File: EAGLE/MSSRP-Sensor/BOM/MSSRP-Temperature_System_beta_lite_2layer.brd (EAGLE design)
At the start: 50 x 75 mm, 54 parts, among them J1 POWER_JACKPTH, J4 TE-2-TERMBLOCK, J5 TE-2-TERMBLOCK, U1 MBED, U12 LP2989AIM, U2 BLUETOOTH-RN41", U5 SI7020-A10, U7 MAX6675, U8 MAX6675

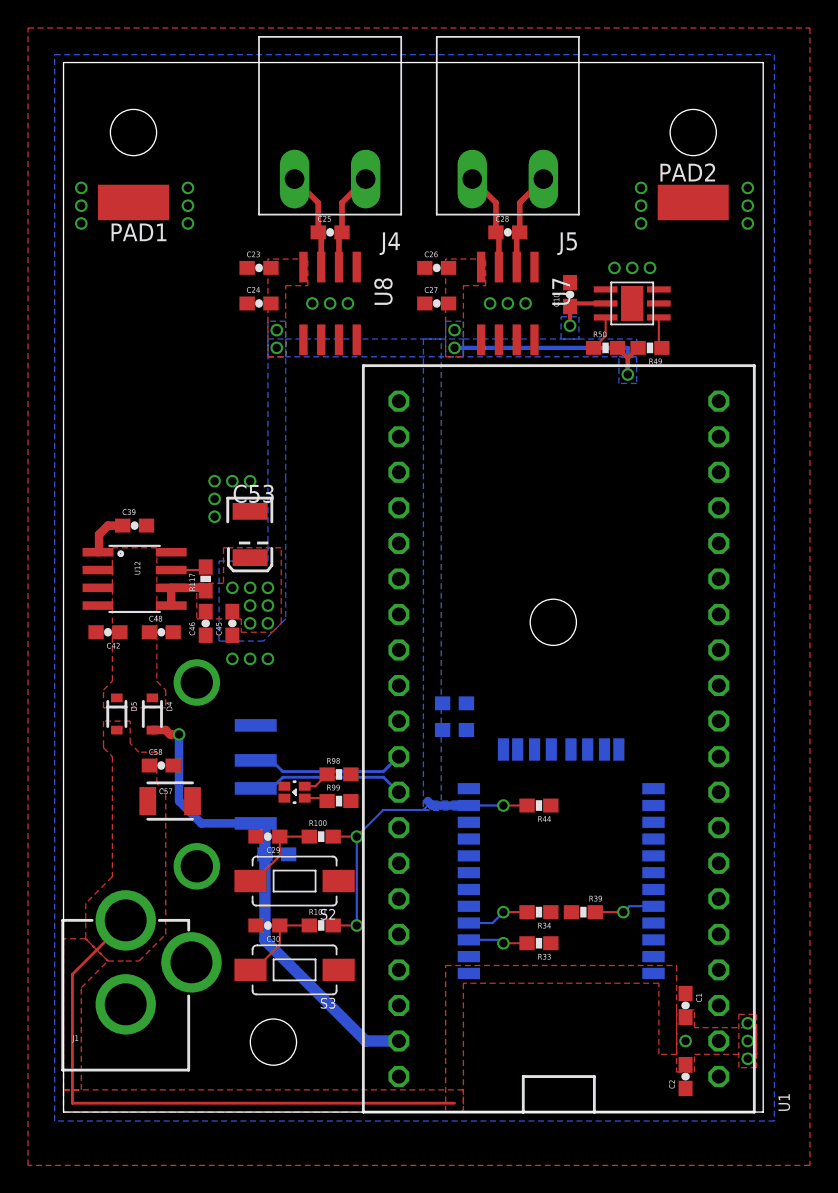
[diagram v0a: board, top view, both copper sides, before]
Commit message: Final Routing
Final routing complete
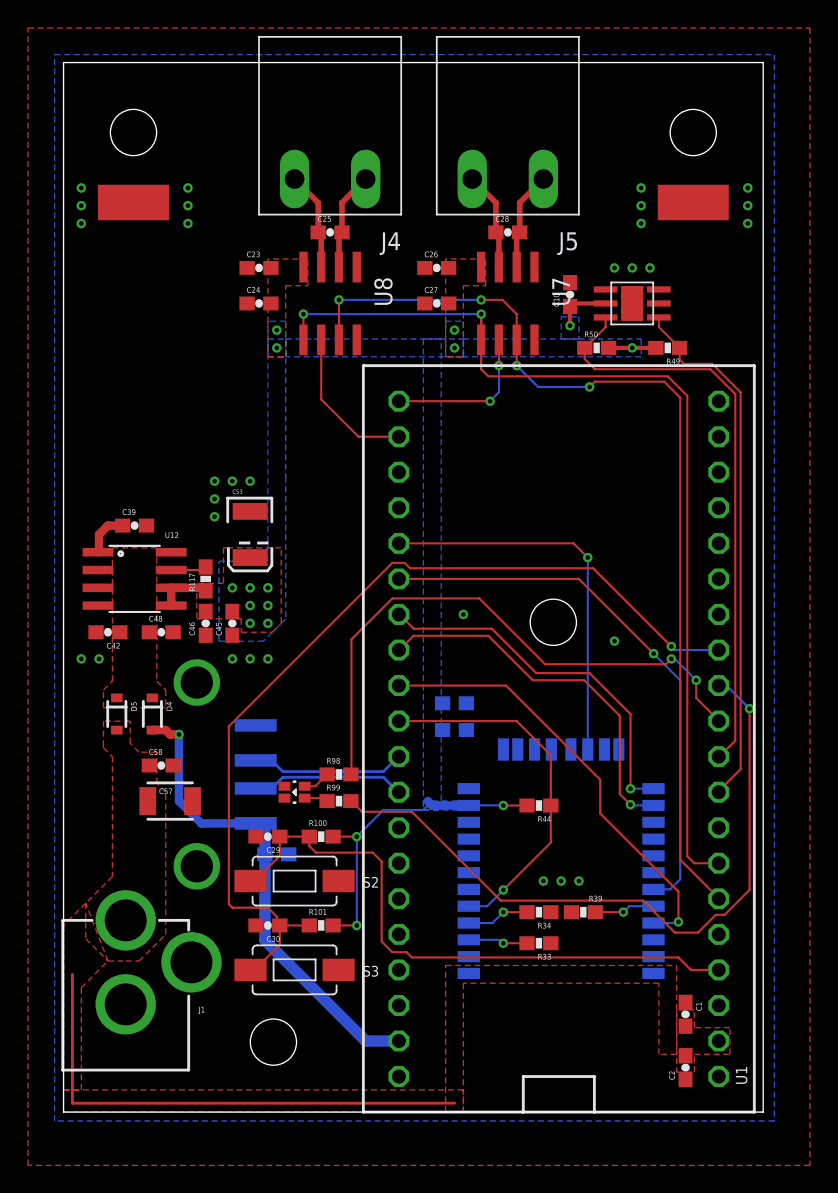
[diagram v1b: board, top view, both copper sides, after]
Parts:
- moved R49 1.27 mm to (43.2, 54.6)
- moved C1 0.63 mm to (44.5, 6.99)
- moved C2 0.63 mm to (44.5, 3.17)
- moved R50 0.63 mm to (38.1, 54.6)
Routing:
- net SCK: track 0.00 -> 70.8 mm, vias 0 -> 2
- net MISO: track 0.00 -> 69.6 mm, vias 0 -> 4
- net SW2: track 6.32 -> 66.0 mm, vias 0 -> 1
- net LED1: track 0.00 -> 49.5 mm, vias 0 -> 1
- net LED0: track 0.00 -> 41.9 mm, vias 0 -> 2
- net BT_CONN: track 0.00 -> 39.5 mm, vias 0 -> 1
- net SCL: track 2.53 -> 41.8 mm
- net MICRO_!RESET: track 6.32 -> 43.3 mm
- net SDA: track 2.27 -> 38.2 mm
- net BT_STATE: track 0.00 -> 31.5 mm, vias 0 -> 1
- net BT_RXTX: track 0.00 -> 27.6 mm, vias 0 -> 1
- net UART_TX: track 0.00 -> 26.9 mm, vias 0 -> 1
- net UART_RX: track 0.00 -> 26.5 mm, vias 0 -> 1
- net BT_RESET: track 0.00 -> 25.9 mm, vias 0 -> 1
- net 3.3V: track 48.6 -> 34.5 mm
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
